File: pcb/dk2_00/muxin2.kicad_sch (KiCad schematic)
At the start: 13 parts, among them J12 AudioJack2_SwitchT, J9 Conn_01x08_Pin, U6 74HC4051, U8 MCP6002-xSN

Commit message: components...
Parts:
- C22, C23: footprint (none) -> Capacitor_SMD:C_0603_1608Metric
- J9: footprint (none) -> Connector_PinHeader_2.54mm:PinHeader_1x08_P2.54mm_Vertical
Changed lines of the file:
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@@
       (effects (font (size 1.27 1.27)))
     )
-    (property "Footprint" "" (at 82.55 26.67 0)
+    (property "Footprint" "Capacitor_SMD:C_0603_1608Metric" (at 82.55 26.67 0)
       (effects (font (size 1.27 1.27)) hide)
     )
@@
       (effects (font (size 1.27 1.27)))
     )
-    (property "Footprint" "" (at 82.55 70.485 0)
+    (property "Footprint" "Capacitor_SMD:C_0603_1608Metric" (at 82.55 70.485 0)
       (effects (font (size 1.27 1.27)) hide)
     )
@@
       (effects (font (size 1.27 1.27)) (justify right))
     )
-    (property "Footprint" "" (at 201.93 98.425 0)
-      (effects (font (size 1.27 1.27)) hide)
-    )
+    (property "Footprint" "Connector_PinHeader_2.54mm:PinHeader_1x08_P2.54mm_Vertical" (at 201.93 98.425 0)
+      (effects (font (size 1.27 1.27)) hide)
+    )

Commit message: footprints assigned
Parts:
- R30, R31, R32, R33, R34, R35: footprint (none) -> Resistor_SMD:R_0603_1608Metric
- U8: footprint (none) -> Package_SO:SOIC-8_3.9x4.9mm_P1.27mm
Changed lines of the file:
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@@
       (effects (font (size 1.27 1.27)))
     )
-    (property "Footprint" "" (at 72.009 78.994 90)
+    (property "Footprint" "Resistor_SMD:R_0603_1608Metric" (at 72.009 78.994 90)
       (effects (font (size 1.27 1.27)) hide)
     )
@@
       (effects (font (size 1.27 1.27)))
     )
-    (property "Footprint" "" (at 83.185 48.895 0)
+    (property "Footprint" "Package_SO:SOIC-8_3.9x4.9mm_P1.27mm" (at 83.185 48.895 0)
       (effects (font (size 1.27 1.27)) hide)
     )
@@
       (effects (font (size 1.27 1.27)))
     )
-    (property "Footprint" "" (at 82.804 78.994 90)
+    (property "Footprint" "Resistor_SMD:R_0603_1608Metric" (at 82.804 78.994 90)
       (effects (font (size 1.27 1.27)) hide)
     )
@@
       (effects (font (size 1.27 1.27)))
     )
-    (property "Footprint" "" (at 83.185 92.71 0)
+    (property "Footprint" "Package_SO:SOIC-8_3.9x4.9mm_P1.27mm" (at 83.185 92.71 0)
       (effects (font (size 1.27 1.27)) hide)
     )
@@
       (effects (font (size 1.27 1.27)))
     )
-    (property "Footprint" "" (at 72.009 35.179 90)
+    (property "Footprint" "Resistor_SMD:R_0603_1608Metric" (at 72.009 35.179 90)
       (effects (font (size 1.27 1.27)) hide)
     )
@@
       (effects (font (size 1.27 1.27)) (justify left))
     )
-    (property "Footprint" "" (at 78.74 123.825 0)
+    (property "Footprint" "Package_SO:SOIC-8_3.9x4.9mm_P1.27mm" (at 78.74 123.825 0)
       (effects (font (size 1.27 1.27)) hide)
     )
@@
       (effects (font (size 1.27 1.27)))
     )
-    (property "Footprint" "" (at 72.009 45.339 90)
+    (property "Footprint" "Resistor_SMD:R_0603_1608Metric" (at 72.009 45.339 90)
       (effects (font (size 1.27 1.27)) hide)
     )
@@
       (effects (font (size 1.27 1.27)))
     )
-    (property "Footprint" "" (at 72.009 89.154 90)
+    (property "Footprint" "Resistor_SMD:R_0603_1608Metric" (at 72.009 89.154 90)
       (effects (font (size 1.27 1.27)) hide)
     )
@@
       (effects (font (size 1.27 1.27)))
     )
-    (property "Footprint" "" (at 82.804 35.179 90)
-      (effects (font (size 1.27 1.27)) hide)
-    )
+    (property "Footprint" "Resistor_SMD:R_0603_1608Metric" (at 82.804 35.179 90)
+      (effects (font (size 1.27 1.27)) hide)
+    )

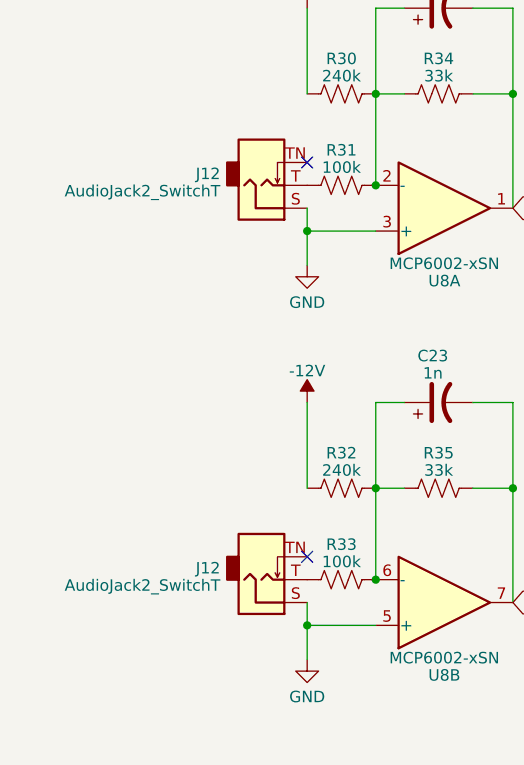
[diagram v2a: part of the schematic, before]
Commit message: this layout is complicated!
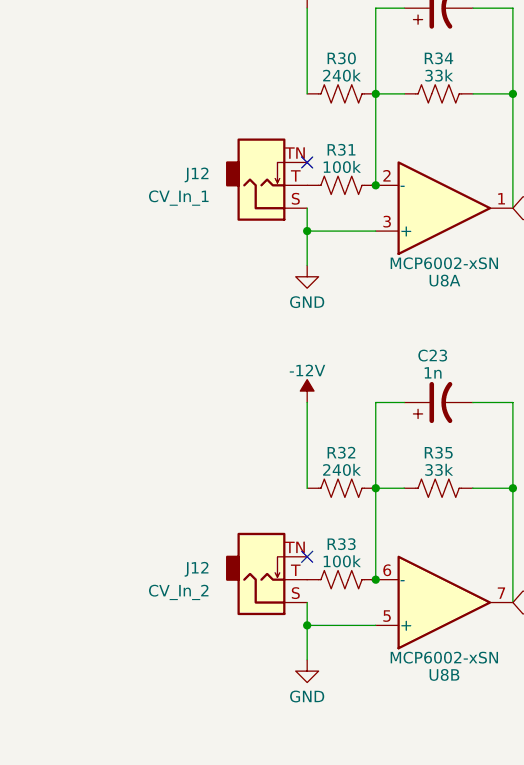
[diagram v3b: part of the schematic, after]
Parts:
- J12: value AudioJack2_SwitchT -> CV_In_2
- J12: value AudioJack2_SwitchT -> CV_In_1
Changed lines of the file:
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@@
   (symbol (lib_id "Connector_Audio:AudioJack2_SwitchT") (at 62.865 90.17 0) (mirror x) (unit 1)
     (in_bom yes) (on_board yes) (dnp no) (fields_autoplaced)
-    (property "Reference" "J12" (at 58.293 88.8913 0)
+    (property "Reference" "J12" (at 57.15 88.9 0)
       (effects (font (size 1.27 1.27)) (justify right))
     )
-    (property "Value" "AudioJack2_SwitchT" (at 58.293 90.8123 0)
+    (property "Value" "CV_In_2" (at 57.15 91.44 0)
       (effects (font (size 1.27 1.27)) (justify right))
     )
@@
   (symbol (lib_id "Connector_Audio:AudioJack2_SwitchT") (at 62.865 46.355 0) (mirror x) (unit 1)
     (in_bom yes) (on_board yes) (dnp no) (fields_autoplaced)
-    (property "Reference" "J12" (at 58.293 45.0763 0)
+    (property "Reference" "J12" (at 57.15 45.085 0)
       (effects (font (size 1.27 1.27)) (justify right))
     )
-    (property "Value" "AudioJack2_SwitchT" (at 58.293 46.9973 0)
+    (property "Value" "CV_In_1" (at 57.15 47.625 0)
       (effects (font (size 1.27 1.27)) (justify right))
     )

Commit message: it's jlc time
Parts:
- J12: footprint AudioJacks:Jack_3.5mm_QingPu_WQP-PJ398SM_Vertical -> Library:Jack_3.5mm_QingPu_WQP-PJ398SM_Vertical_Labelled
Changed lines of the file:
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@@
       (effects (font (size 1.27 1.27)) (justify right))
     )
-    (property "Footprint" "AudioJacks:Jack_3.5mm_QingPu_WQP-PJ398SM_Vertical" (at 62.865 90.17 0)
+    (property "Footprint" "Library:Jack_3.5mm_QingPu_WQP-PJ398SM_Vertical_Labelled" (at 62.865 90.17 0)
       (effects (font (size 1.27 1.27)) hide)
     )
@@
       (effects (font (size 1.27 1.27)) (justify right))
     )
-    (property "Footprint" "AudioJacks:Jack_3.5mm_QingPu_WQP-PJ398SM_Vertical" (at 62.865 46.355 0)
+    (property "Footprint" "Library:Jack_3.5mm_QingPu_WQP-PJ398SM_Vertical_Labelled" (at 62.865 46.355 0)
       (effects (font (size 1.27 1.27)) hide)
     )
